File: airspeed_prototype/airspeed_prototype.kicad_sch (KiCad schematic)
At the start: 6 parts, among them J1 Conn_01x03_Pin, J3 Conn_01x06_Pin, J4 Conn_01x08_Pin, U1 ESP32-DevKitC

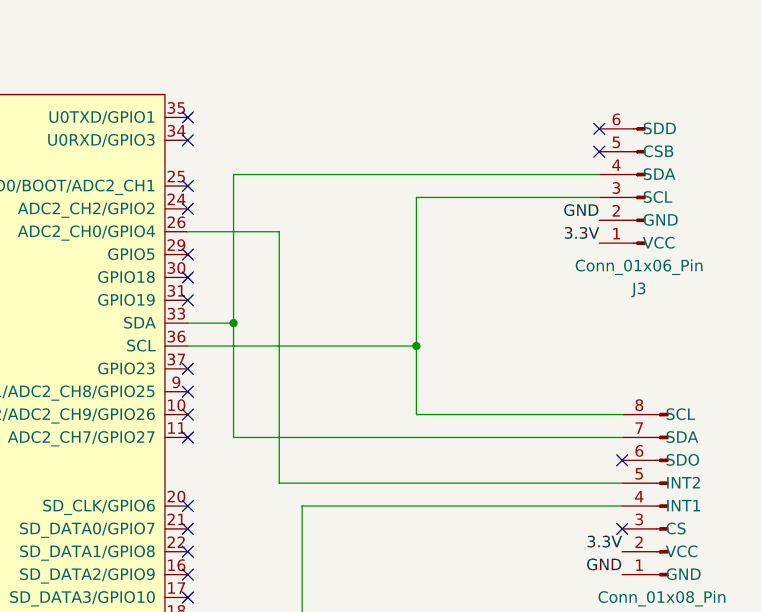
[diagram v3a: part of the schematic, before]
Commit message: updates to pcb
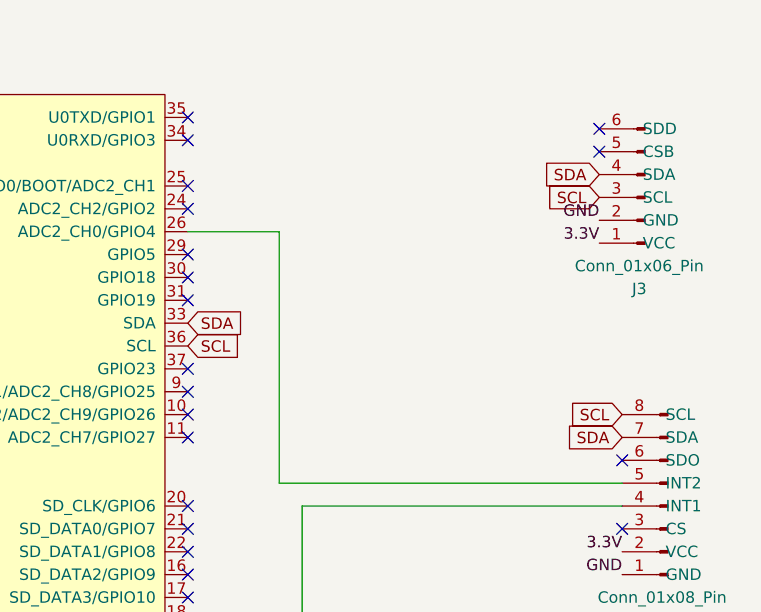
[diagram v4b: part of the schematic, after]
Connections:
- net SDA: now reaches J3.4 (SDA), J4.7 (SDA), U1.33 (GPIO21)
- net SCL: now reaches J3.3 (SCL), J4.8 (SCL), U1.36 (GPIO22)
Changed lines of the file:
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@@
   (junction (at 68.58 55.88) (diameter 0) (color 0 0 0 0)
-  )
-  (junction (at 200.66 73.66) (diameter 0) (color 0 0 0 0)
-  )
-  (junction (at 220.98 76.2) (diameter 0) (color 0 0 0 0)
   )
   (junction (at 68.58 88.9) (diameter 0) (color 0 0 0 0)
@@
     (stroke (width 0) (type default))
   )
-  (wire (pts (xy 241.3 59.69) (xy 220.98 59.69))
-    (stroke (width 0) (type default))
-  )
   (wire (pts (xy 68.58 67.31) (xy 68.58 88.9))
     (stroke (width 0) (type default))
@@
     (stroke (width 0) (type default))
   )
-  (wire (pts (xy 243.84 83.82) (xy 220.98 83.82))
-    (stroke (width 0) (type default))
-  )
   (wire (pts (xy 129.54 55.88) (xy 68.58 55.88))
     (stroke (width 0) (type default))
   )
   (wire (pts (xy 162.56 116.84) (xy 162.56 132.08))
-    (stroke (width 0) (type default))
-  )
-  (wire (pts (xy 220.98 76.2) (xy 195.58 76.2))
     (stroke (width 0) (type default))
   )
@@
     (stroke (width 0) (type default))
   )
-  (wire (pts (xy 200.66 57.15) (xy 200.66 73.66))
-    (stroke (width 0) (type default))
-  )
   (wire (pts (xy 205.74 91.44) (xy 205.74 63.5))
     (stroke (width 0) (type default))
@@
     (stroke (width 0) (type default))
   )
-  (wire (pts (xy 200.66 86.36) (xy 243.84 86.36))
-    (stroke (width 0) (type default))
-  )
   (wire (pts (xy 172.72 45.72) (xy 165.1 45.72))
     (stroke (width 0) (type default))
   )
   (wire (pts (xy 68.58 50.8) (xy 68.58 55.88))
-    (stroke (width 0) (type default))
-  )
-  (wire (pts (xy 241.3 57.15) (xy 200.66 57.15))
     (stroke (width 0) (type default))
   )
@@
     (stroke (width 0) (type default))
   )
-  (wire (pts (xy 220.98 59.69) (xy 220.98 76.2))
-    (stroke (width 0) (type default))
-  )
   (wire (pts (xy 68.58 55.88) (xy 68.58 59.69))
     (stroke (width 0) (type default))
   )
   (wire (pts (xy 68.58 43.18) (xy 68.58 38.1))
-    (stroke (width 0) (type default))
-  )
-  (wire (pts (xy 200.66 73.66) (xy 195.58 73.66))
-    (stroke (width 0) (type default))
-  )
-  (wire (pts (xy 220.98 83.82) (xy 220.98 76.2))
-    (stroke (width 0) (type default))
-  )
-  (wire (pts (xy 200.66 73.66) (xy 200.66 86.36))
     (stroke (width 0) (type default))
   )
@@
     (effects (font (size 1.27 1.27)) (justify left bottom))
   )
+  (global_label "SDA" (shape input) (at 241.3 57.15 180) (fields_autoplaced)
+    (effects (font (size 1.27 1.27)) (justify right))
+    (property "Intersheetrefs" "${INTERSHEET_REFS}" (at 234.7467 57.15 0)
+      (effects (font (size 1.27 1.27)) (justify right) hide)
+    )
+  )
+  (global_label "SDA" (shape input) (at 243.84 86.36 180) (fields_autoplaced)
+    (effects (font (size 1.27 1.27)) (justify right))
+    (property "Intersheetrefs" "${INTERSHEET_REFS}" (at 237.2867 86.36 0)
+      (effects (font (size 1.27 1.27)) (justify right) hide)
+    )
+  )
+  (global_label "SDA" (shape input) (at 195.58 73.66 0) (fields_autoplaced)
+    (effects (font (size 1.27 1.27)) (justify left))
+    (property "Intersheetrefs" "${INTERSHEET_REFS}" (at 202.1333 73.66 0)
+      (effects (font (size 1.27 1.27)) (justify left) hide)
+    )
+  )
+  (global_label "SCL" (shape input) (at 241.3 59.69 180) (fields_autoplaced)
+    (effects (font (size 1.27 1.27)) (justify right))
+    (property "Intersheetrefs" "${INTERSHEET_REFS}" (at 234.8072 59.69 0)
+      (effects (font (size 1.27 1.27)) (justify right) hide)
+    )
+  )
+  (global_label "SCL" (shape input) (at 195.58 76.2 0) (fields_autoplaced)
+    (effects (font (size 1.27 1.27)) (justify left))
+    (property "Intersheetrefs" "${INTERSHEET_REFS}" (at 202.0728 76.2 0)
+      (effects (font (size 1.27 1.27)) (justify left) hide)
+    )
+  )
+  (global_label "SCL" (shape input) (at 243.84 83.82 180) (fields_autoplaced)
+    (effects (font (size 1.27 1.27)) (justify right))
+    (property "Intersheetrefs" "${INTERSHEET_REFS}" (at 237.3472 83.82 0)
+      (effects (font (size 1.27 1.27)) (justify right) hide)
+    )
+  )
   (symbol (lib_id "power:GND") (at 68.58 88.9 0) (unit 1)
